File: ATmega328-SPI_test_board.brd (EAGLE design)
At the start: 99.1 x 80 mm, 55 parts, among them J1 DC jack, J2 USB mini, SW1 Power switch

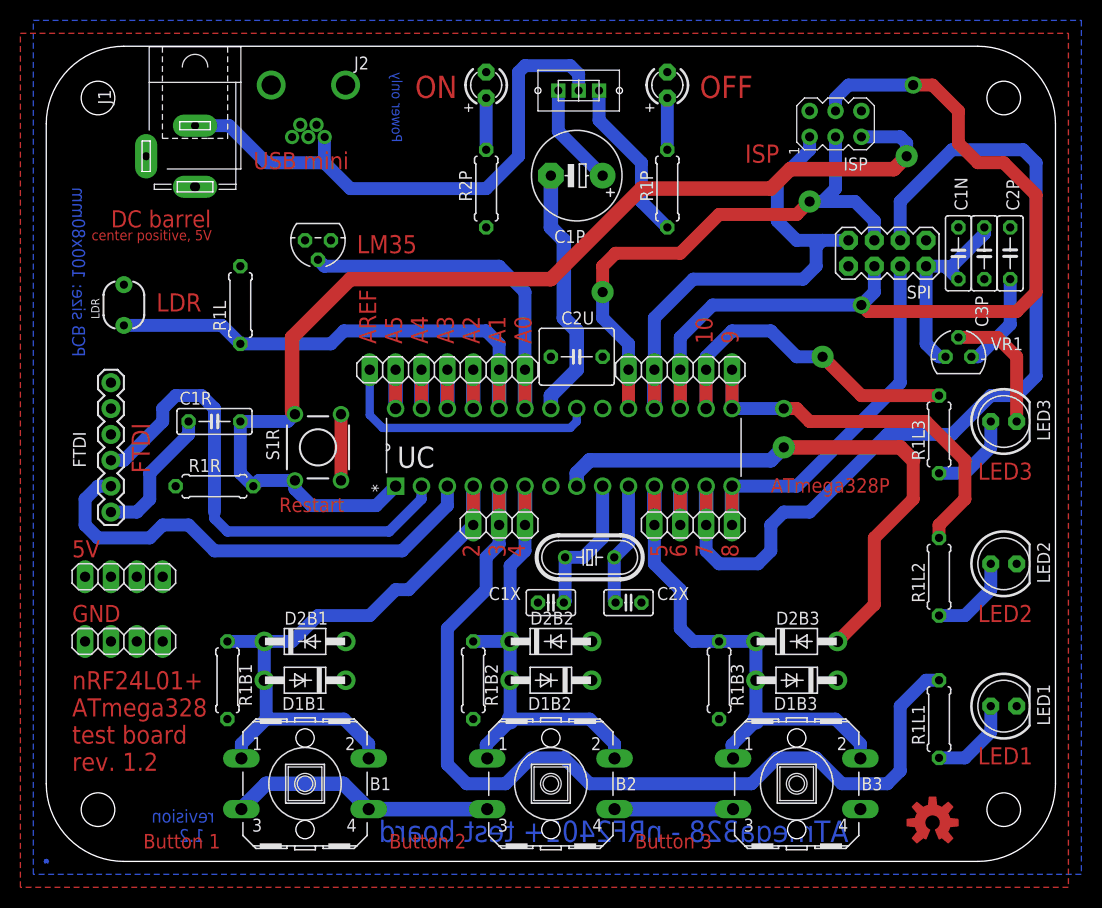
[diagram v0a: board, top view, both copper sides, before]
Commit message: Corrections
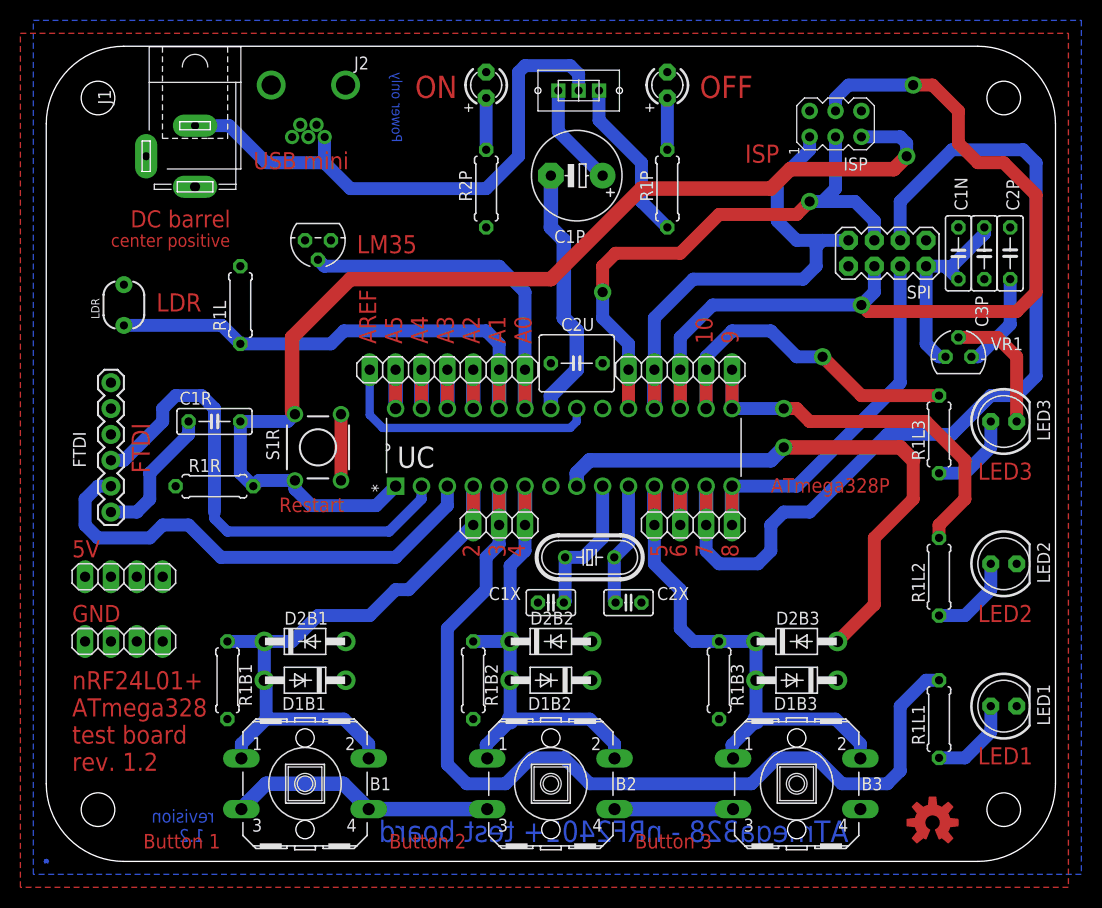
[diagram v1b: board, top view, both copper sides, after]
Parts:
- moved C2U 0.63 mm to (52.1, 48.9)
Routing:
- net UTX: track 47.0 -> 47.5 mm
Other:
- board text added: "center positive"
- board text removed: "PCB size: 100x80mm"
- board text removed: "center positive, 5V"
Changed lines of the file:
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@@
 <text x="16.51" y="1.905" size="1.27" layer="16" font="vector" rot="MR0">revision
   1.2</text>
-<text x="6.35" y="62.23" size="1.6764" layer="1" font="vector">DC barrel</text>
-<text x="4.445" y="60.96" size="1.016" layer="1" font="vector">center positive, 5V</text>
+<text x="8.255" y="62.23" size="1.6764" layer="1" font="vector">DC barrel</text>
+<text x="6.35" y="60.325" size="1.27" layer="1" font="vector">center positive</text>
 <text x="34.925" y="77.47" size="1.016" layer="16" font="vector" rot="MR270">Power only</text>
-<text x="2.54" y="49.53" size="1.27" layer="16" font="vector" rot="MR90">PCB size: 100x80mm</text>
 </plain>
 <attributes>
@@
 <attribute name="VALUE" x="86.741" y="63.119" size="1.27" layer="27" ratio="10" rot="R270"/>
 </element>
-<element name="C2U" library="rcl" package="C050-055X075" value="" x="52.07" y="49.53" smashed="yes" rot="R180">
-<attribute name="NAME" x="50.546" y="52.705" size="1.27" layer="25" ratio="10"/>
-<attribute name="VALUE" x="55.372" y="51.816" size="1.27" layer="27" ratio="10" rot="R180"/>
+<element name="C2U" library="rcl" package="C050-055X075" value="" x="52.07" y="48.895" smashed="yes" rot="R180">
+<attribute name="NAME" x="50.546" y="52.07" size="1.27" layer="25" ratio="10"/>
+<attribute name="VALUE" x="55.372" y="51.181" size="1.27" layer="27" ratio="10" rot="R180"/>
 </element>
 <element name="B1" library="switch-omron" package="B3F-40XX" value="" x="25.4" y="7.62" smashed="yes">
@@
 <wire x1="53.34" y1="39.37" x2="71.12" y2="39.37" width="1.4224" layer="16"/>
 <wire x1="71.12" y1="39.37" x2="72.39" y2="40.64" width="1.4224" layer="16"/>
-<via x="72.39" y="40.64" extent="1-16" drill="1" diameter="2.1844" shape="square"/>
+<via x="72.39" y="40.64" extent="1-16" drill="1" shape="square"/>
 <wire x1="72.39" y1="40.64" x2="83.82" y2="40.64" width="1.4224" layer="1"/>
 <wire x1="83.82" y1="40.64" x2="85.09" y2="39.37" width="1.4224" layer="1"/>
@@
 <wire x1="73.025" y1="67.945" x2="83.185" y2="67.945" width="1.4224" layer="1"/>
 <wire x1="83.185" y1="67.945" x2="84.455" y2="69.215" width="1.4224" layer="1"/>
-<via x="84.455" y="69.215" extent="1-16" drill="1" diameter="2.1844" shape="square"/>
+<via x="84.455" y="69.215" extent="1-16" drill="1" shape="square"/>
 <wire x1="84.455" y1="69.215" x2="84.455" y2="70.485" width="1.27" layer="16"/>
 <wire x1="84.455" y1="70.485" x2="83.82" y2="71.12" width="1.27" layer="16"/>
@@
 <wire x1="10.16" y1="31.75" x2="11.43" y2="33.02" width="1.27" layer="16"/>
 <wire x1="11.43" y1="33.02" x2="13.97" y2="33.02" width="1.27" layer="16"/>
-<wire x1="13.97" y1="33.02" x2="16.51" y2="30.48" width="1.27" layer="16"/>
-<wire x1="16.51" y1="30.48" x2="34.925" y2="30.48" width="1.27" layer="16"/>
-<wire x1="34.925" y1="30.48" x2="39.37" y2="34.925" width="1.27" layer="16"/>
+<wire x1="13.97" y1="33.02" x2="17.145" y2="29.845" width="1.27" layer="16"/>
+<wire x1="34.29" y1="29.845" x2="39.37" y2="34.925" width="1.27" layer="16"/>
 <wire x1="39.37" y1="34.925" x2="39.37" y2="36.83" width="1.27" layer="16"/>
+<wire x1="17.145" y1="29.845" x2="34.29" y2="29.845" width="1.27" layer="16"/>
 </signal>
 <signal name="N$7">
@@
 <contactref element="H3U" pad="5"/>
 <wire x1="57.15" y1="44.45" x2="57.15" y2="48.26" width="1.27" layer="16"/>
-<via x="54.61" y="55.88" extent="1-16" drill="1" diameter="2.1844" shape="square"/>
+<via x="54.61" y="55.88" extent="1-16" drill="1" shape="square"/>
 <wire x1="54.61" y1="55.88" x2="54.61" y2="53.34" width="1.27" layer="16"/>
 <wire x1="54.61" y1="53.34" x2="57.15" y2="50.8" width="1.27" layer="16"/>
 <wire x1="57.15" y1="50.8" x2="57.15" y2="48.26" width="1.27" layer="16"/>
-<via x="74.93" y="64.77" extent="1-16" drill="1" diameter="2.1844" shape="square"/>
+<via x="74.93" y="64.77" extent="1-16" drill="1" shape="square"/>
 <wire x1="74.93" y1="64.77" x2="76.2" y2="64.77" width="1.27" layer="16"/>
 <wire x1="76.2" y1="64.77" x2="77.47" y2="66.04" width="1.27" layer="16"/>
@@
 <contactref element="R1L3" pad="2"/>
 <wire x1="64.77" y1="48.26" x2="64.77" y2="44.45" width="1.27" layer="16"/>
-<via x="76.2" y="49.53" extent="1-16" drill="1" diameter="2.1844" shape="square"/>
+<via x="76.2" y="49.53" extent="1-16" drill="1" shape="square"/>
 <wire x1="76.2" y1="49.53" x2="73.66" y2="49.53" width="1.27" layer="16"/>
 <wire x1="73.66" y1="49.53" x2="71.12" y2="52.07" width="1.27" layer="16"/>
